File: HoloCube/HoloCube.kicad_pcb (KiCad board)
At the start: 4 copper layers, 60.4 x 50 mm, 40 parts, among them J1 ESPProgUART_RX, J2 Conn_01x08_MountingPin, J3 USB_C_Receptacle_USB2.0, J4 Micro_SD_Card, J5 ESPProgJTAG_RX, U1 ESP32-PICO-D4, U2 LIS2DH12TR, U3 BH1750FVI-TR, U4 XC6209

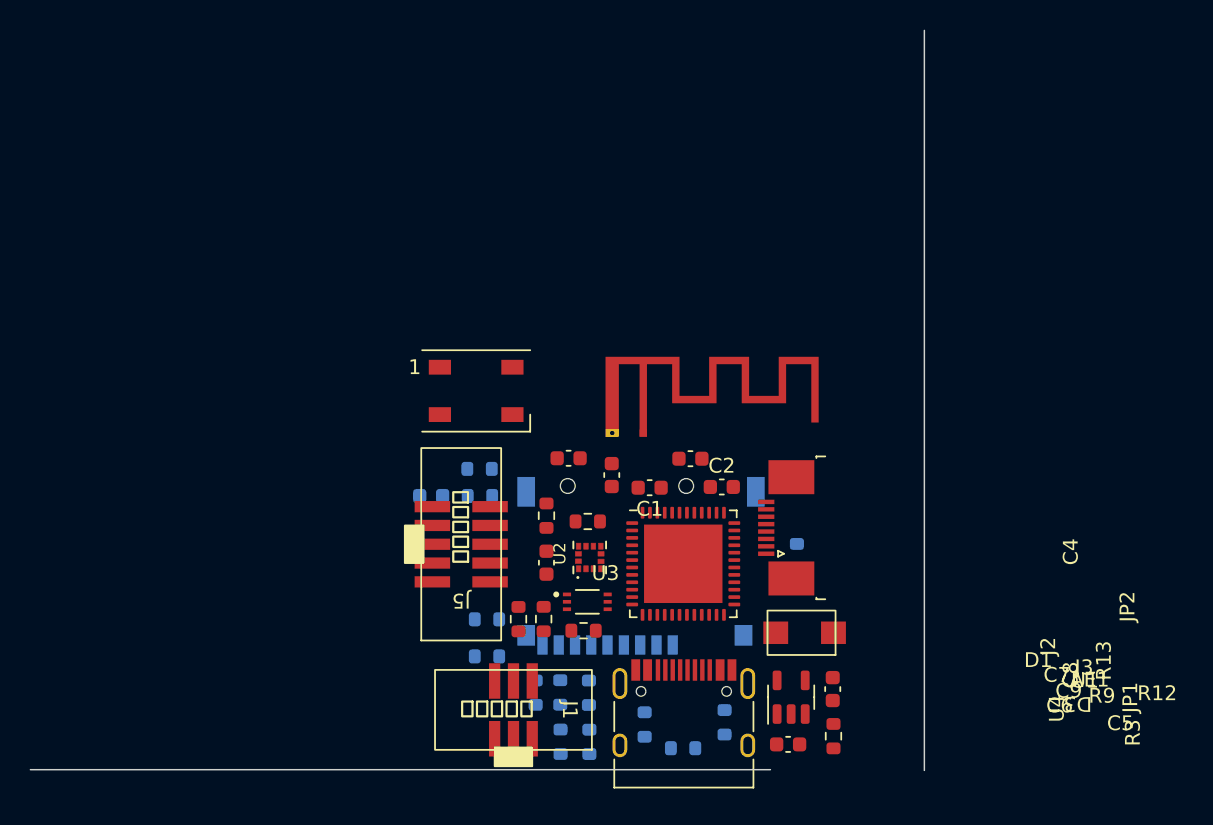
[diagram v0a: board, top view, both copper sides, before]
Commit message: Random Version 0.0
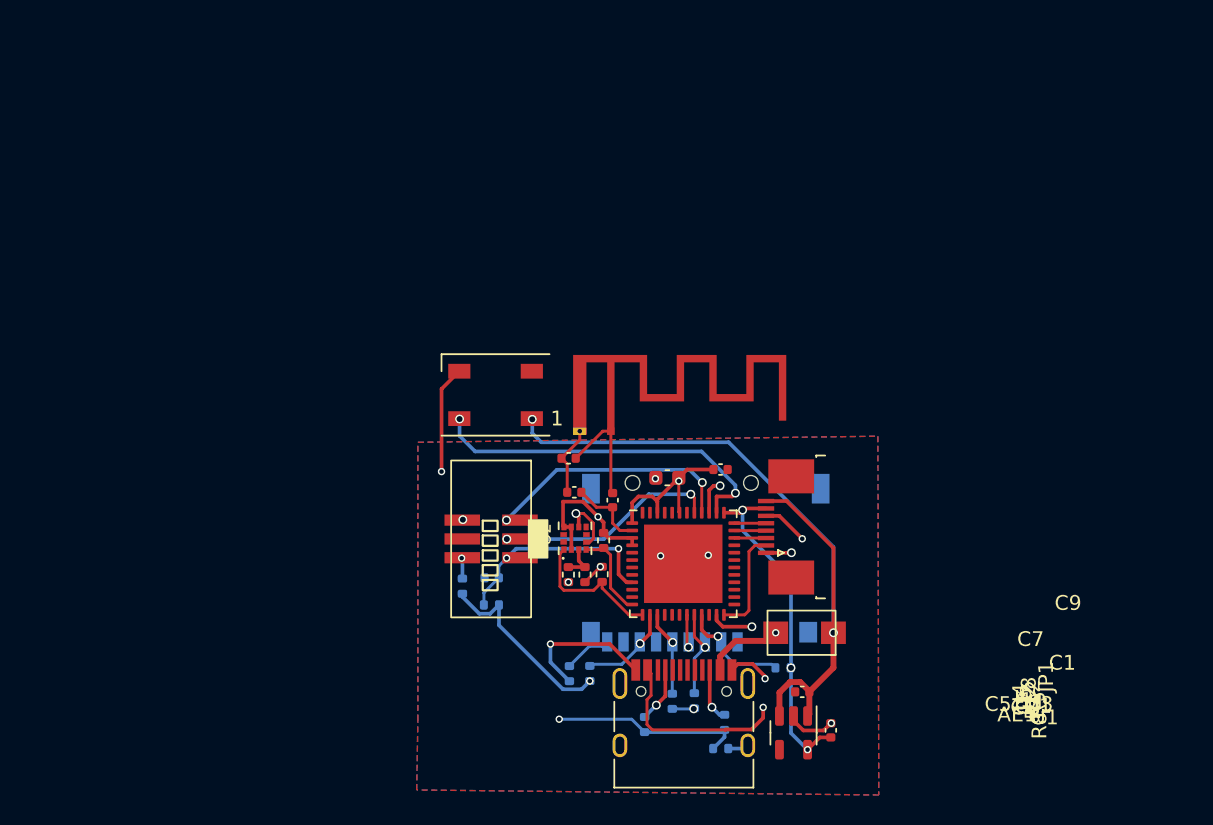
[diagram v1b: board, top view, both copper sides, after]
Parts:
- removed C4: 0.1uf, Capacitor_SMD:C_0603_1608Metric
- removed J5: ESPProgJTAG_RX, KisonNew:IDC_1.27mm_10P
- removed JP2: Jumper, Resistor_SMD:R_0603_1608Metric
- removed R10, R9: 10k, Resistor_SMD:R_0603_1608Metric
- removed R13: 100k, Resistor_SMD:R_0603_1608Metric
- removed R3: 0, Resistor_SMD:R_0603_1608Metric
- removed U3: BH1750FVI-TR, BH1750FVI-TR:XDCR_BH1750FVI-TR
- C2, C3, C5, C6, C7, C8, C9: footprint Capacitor_SMD:C_0603_1608Metric -> Capacitor_SMD:C_0402_1005Metric
- JP1, R1, R11, R12, R14, R15, R16, R17, R2, R4, R6, R7: footprint Resistor_SMD:R_0603_1608Metric -> Resistor_SMD:R_0402_1005Metric
- R5, R8: footprint Resistor_SMD:R_0603_1608Metric -> Resistor_SMD:R_0402_1005Metric; moved to F.Cu
- moved R17 14.0 mm to (215.5, 123.1), turned to 180 degrees
- moved J1 11.6 mm to (195.8, 114.4), turned to -90 degrees
- moved R8 11.1 mm to (203.4, 114.5), turned to -90 degrees
- moved R15 9.46 mm to (209.5, 125.3), turned to 90 degrees
- moved R5 8.35 mm to (203.3, 116.8), turned to -90 degrees
- moved C7 8.17 mm to (201.4, 111.3), turned to 0 degrees
- moved R2 8.00 mm to (193.8, 117.6), turned to 90 degrees
- moved R1 7.40 mm to (195.8, 118.9)
- moved C3 6.88 mm to (195.8, 117.0)
- moved R16 5.66 mm to (208.0, 125.4)
- moved J4 4.38 mm to (209.7, 115.5)
- moved JP1 4.25 mm to (201.0, 116.8)
- moved C5 3.68 mm to (216.8, 124.7)
- moved R12 3.60 mm to (202.1, 116.8), turned to -90 degrees
- moved C6 2.79 mm to (218.7, 127.3), turned to 90 degrees
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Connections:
- AE1 pad 2: (no net) -> GND
- C1 pad 1: +3.3VA -> +3V3
- C2 pad 1: +3.3VA -> +3V3
- D1 pad 4: /IO27 -> /IO19
- J2 pad 1: /IO5 -> /IO22
- J2 pad 3: /IO23 -> /IO5
- J4 pad 2: /IO21 -> /IO15
- J4 pad 3: /IO25 -> /IO13
- J4 pad 5: /IO19 -> /IO26
- J4 pad 7: /IO26 -> /IO25
- R14 pad 2: /IO26 -> /IO25
- R15 pad 2: /IO25 -> /IO13
- R16 pad 2: /IO19 -> /IO26
- R17 pad 2: /IO21 -> /IO15
- R2 pad 1: Net-(J1-Pad2) -> +3V3
- R2 pad 2: +3V3 -> Net-(J1-Pad2)
- U1 pad 1: +3.3VA -> +3V3
- U1 pad 18: /TDI -> /IO12
- U1 pad 19: +3.3VA -> +3V3
- U1 pad 20: /TCLK -> /IO13
- U1 pad 21: /TDO -> /IO15
- U1 pad 22: /DC -> unconnected-(U1-Pad22)
- U1 pad 3: +3.3VA -> +3V3
- U1 pad 36: /IO23 -> /DC
- U1 pad 37: +3.3VA -> +3V3
- U1 pad 4: +3.3VA -> +3V3
- U1 pad 42: /IO21 -> unconnected-(U1-Pad42)
- U1 pad 43: +3.3VA -> +3V3
- U1 pad 46: +3.3VA -> +3V3
- U2 pad 6: GND -> unconnected-(U2-Pad6)
- U2 pad 7: GND -> unconnected-(U2-Pad7)
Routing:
- net +3V3: track 0.00 -> 99.4 mm, vias 0 -> 9
- net GND: track 0.00 -> 73.0 mm, vias 0 -> 11
- net +5V: track 0.00 -> 52.4 mm, vias 0 -> 2
- net /IO0: track 0.00 -> 25.7 mm, vias 0 -> 2
- net /IO19: track 0.00 -> 24.2 mm, vias 0 -> 2
- net Net-(D3-Pad2): track 0.00 -> 23.7 mm, vias 0 -> 2
- net Net-(J3-PadS1): track 0.00 -> 18.4 mm
- net /RX: track 0.00 -> 17.1 mm, vias 0 -> 2
- net /IO22: track 0.00 -> 15.4 mm, vias 0 -> 2
- net /TX: track 0.00 -> 15.0 mm, vias 0 -> 2
- net /EN: track 0.00 -> 14.5 mm, vias 0 -> 2
- net /I2C_SCL: track 0.00 -> 9.69 mm
- net /IO15: track 0.00 -> 7.84 mm, vias 0 -> 1
- net Net-(AE1-Pad1): track 0.00 -> 7.36 mm
- net /IO4: track 0.00 -> 7.13 mm
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- added copper zone on B.Cu, net GND
- added copper zone on F.Cu, net GND
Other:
- board outline removed
